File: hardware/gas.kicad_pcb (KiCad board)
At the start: 2 copper layers, 65 x 30 mm, 29 parts, among them P1 CON-SENSOR2, P2 DEBUG, P3 BOOT, P4 Gas Sensor, U1 XMC1300, U2 DRILL, U3 DRILL, U4 DRILL, U5 DRILL

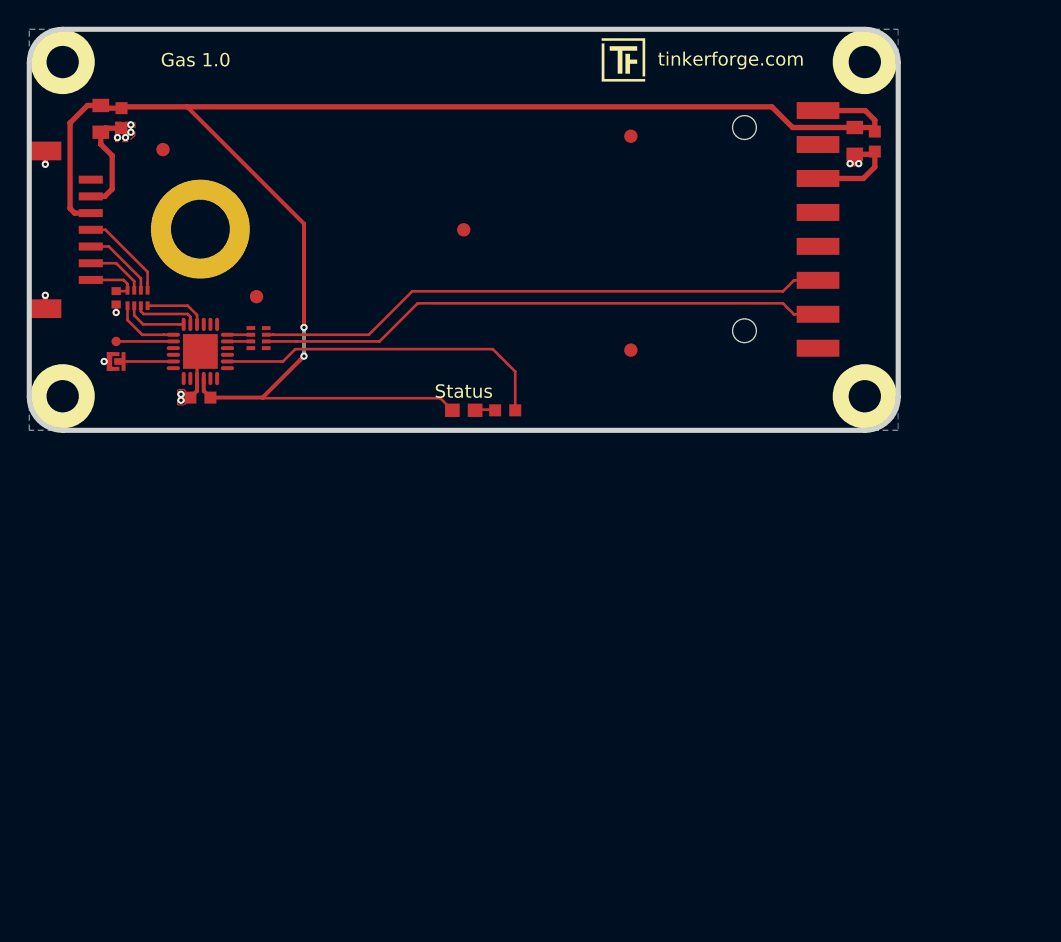
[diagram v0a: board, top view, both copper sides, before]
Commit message: all new design
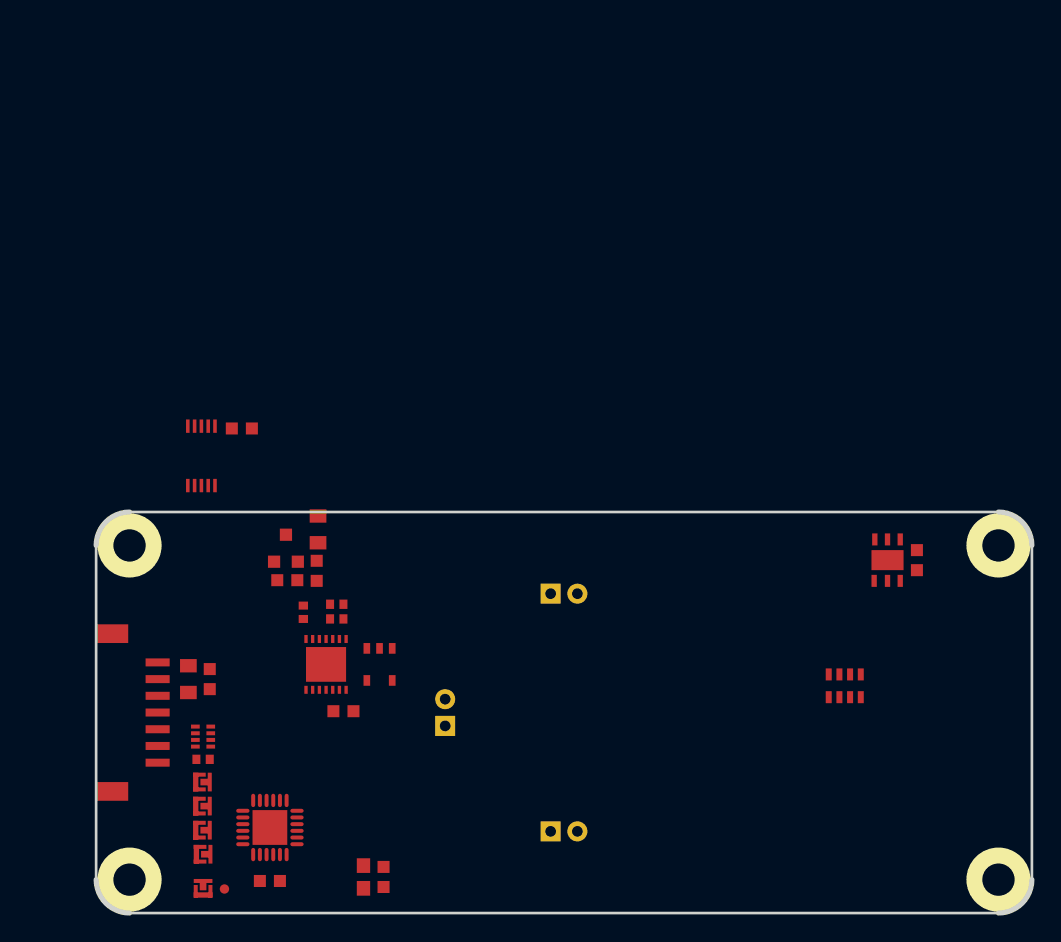
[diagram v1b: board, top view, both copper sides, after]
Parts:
- removed Fiducial_Mark (x5): VAL**, kicad-libraries:Fiducial_Mark
- removed G***: LOGO, kicad-libraries:Logo_31x31
- removed G***: LOGO, kicad-libraries:Logo_CoMCU
- removed REF**: WA-SMSI-M3-SPACER, kicad-libraries:WA-SMSI-M3-SPACER
- removed VAL: WEEE_7mm, kicad-libraries:WEEE_7mm
- removed VAL: CE_5mm, kicad-libraries:CE_5mm
- added C10: 100nF, kicad-libraries:C0603F, F.Cu at (135.9, 109.9)
- added C7: 100nF, kicad-libraries:C0603F, F.Cu at (186.4, 119.7)
- added C8: 10uF TPSA106K010R0900, kicad-libraries:C0805P, F.Cu at (141.6, 117.4)
- added C9: DNP, kicad-libraries:R0402F, F.Cu at (143.0, 123.0)
- added P10: 3, kicad-libraries:SolderJumper, F.Cu at (133.0, 141.7)
- added P5: WORK, kicad-libraries:THT-2-2mm, F.Cu at (160.0, 140.0)
- added P6: GND, kicad-libraries:THT-2-2mm, F.Cu at (151.1, 131.1)
- added P7: 0, kicad-libraries:SolderJumper, F.Cu at (132.9, 136.3)
- added P8: 1, kicad-libraries:SolderJumper, F.Cu at (132.9, 138.1)
- added P9: 2, kicad-libraries:SolderJumper, F.Cu at (132.9, 139.9)
- added R2: 1k, kicad-libraries:R0603F, F.Cu at (141.5, 120.5)
- added R3: 499k, kicad-libraries:R0402F, F.Cu at (143.0, 124.1)
- added R4: 49,9, kicad-libraries:R0402F, F.Cu at (140.5, 123.6)
- added U10: MCP3423, kicad-libraries:MSOP10-0.5, F.Cu at (132.9, 111.9)
- added U6: HDC1080, kicad-libraries:DFN6-30x30_humidity, F.Cu at (184.2, 119.7)
- added U7: ISL60002, kicad-libraries:SOT23-3, F.Cu at (139.2, 118.8)
- added U8: LMP91000, kicad-libraries:WSON-14-LMP91000, F.Cu at (142.2, 127.5)
- added U9: MCP6041, kicad-libraries:SOT23-5, F.Cu at (146.2, 127.5)
- C5: value 10uF -> 100nF; footprint kicad-libraries:C0805 -> kicad-libraries:C0603F
- C6: value 100n -> 100nF
- P4: value Gas Sensor -> RC; footprint kicad-libraries:pin_array_8x1_smd -> kicad-libraries:THT-2-2mm
- RP2: value 100 -> 10k; footprint kicad-libraries:4X0402 -> kicad-libraries:0603X4
- moved U3 70.9 mm to (192.5, 118.6)
- moved U5 65.8 mm to (127.5, 118.6)
- moved U2 61.4 mm to (127.5, 143.6)
- moved C5 57.3 mm to (143.5, 131.0), turned to 0 degrees
- moved C6 54.8 mm to (139.3, 121.2), turned to 180 degrees
- moved RP2 51.0 mm to (181.0, 129.1), turned to 0 degrees
- moved C3 42.5 mm to (133.5, 128.6), turned to 270 degrees
- moved C2 42.4 mm to (131.9, 128.6), turned to 270 degrees
- moved P2 41.8 mm to (134.6, 144.3), turned to 0 degrees
- moved P3 39.9 mm to (133.0, 144.3), turned to 90 degrees
- moved U4 37.5 mm to (192.5, 143.6)
- moved C4 36.5 mm to (138.0, 143.7)
- moved P1 36.5 mm to (125.0, 131.1)
- moved R1 36.1 mm to (146.5, 143.4), turned to 90 degrees
- moved U1 36.0 mm to (138.0, 139.7)
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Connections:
- C5 pad 1: GND -> VCC
- C5 pad 2: VCC -> GND
- C6 pad 1: VCC -> Net-(C6-Pad1)
- RP2 pad 1: Net-(RP2-Pad1) -> VCC
- RP2 pad 2: GS_RX -> Net-(RP2-Pad2)
- RP2 pad 3: GS_TX -> Net-(RP2-Pad3)
- RP2 pad 4: Net-(RP2-Pad4) -> VCC
- RP2 pad 5: Net-(RP2-Pad5) -> SCL0
- RP2 pad 6: Net-(P4-Pad2) -> Net-(RP2-Pad6)
- RP2 pad 7: Net-(P4-Pad3) -> Net-(RP2-Pad7)
- RP2 pad 8: Net-(RP2-Pad8) -> SDA0
- U1 pad 17: GS_TX -> SDA0
- U1 pad 18: GS_RX -> Net-(U1-Pad18)
- U1 pad 19: Net-(U1-Pad19) -> SCL0
- U1 pad 2: Net-(P2-Pad1) -> SolderJumper0
- U1 pad 20: Net-(U1-Pad20) -> Enable
- U1 pad 3: Net-(U1-Pad3) -> SolderJumper1
- U1 pad 4: Net-(U1-Pad4) -> SolderJumper2
- U1 pad 5: Net-(P3-Pad2) -> SolderJumper3
- U1 pad 6: Net-(U1-Pad6) -> Net-(P3-Pad2)
- U1 pad 7: Net-(U1-Pad7) -> Net-(P2-Pad1)
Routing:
- net VCC: track 121.9 -> 0.00 mm, vias 2 -> 0
- net Net-(P4-Pad3): track 43.0 -> 0.00 mm
- net Net-(P4-Pad2): track 42.8 -> 0.00 mm
- net GND: track 31.4 -> 0.00 mm, vias 12 -> 0
- net Net-(R1-Pad1): track 25.5 -> 0.00 mm
- net Net-(P1-Pad4): track 7.43 -> 0.00 mm
- net Net-(P1-Pad5): track 5.62 -> 0.00 mm
- net S-MISO: track 4.96 -> 0.00 mm
- net S-CLK: track 4.87 -> 0.00 mm
- net Net-(C1-Pad1): track 4.83 -> 0.00 mm
- net S-MOSI: track 4.70 -> 0.00 mm
- net S-CS: track 4.69 -> 0.00 mm
- net Net-(P1-Pad6): track 4.48 -> 0.00 mm
- net Net-(P2-Pad1): track 4.33 -> 0.00 mm
- net Net-(P3-Pad2): track 4.12 -> 0.00 mm
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- removed copper zone on B.Cu, net GND
- removed copper zone on F.Cu, net GND
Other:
- board size 65 x 30 mm -> 70 x 30 mm
- net class Default: clearance 0.149 -> 0.2
- rule trace_clearance: 0.149 -> 0.2
- rule trace_min: 0.1 -> 0.2
- rule via_min_drill: 0.25 -> 0.3
- board text removed: "Gas 1.0"
- board text removed: "Status"
- board text removed: "tinkerforge.com"
